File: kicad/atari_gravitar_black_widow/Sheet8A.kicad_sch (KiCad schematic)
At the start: 89 parts, among them Q11 2N3906, Q12 2N3904

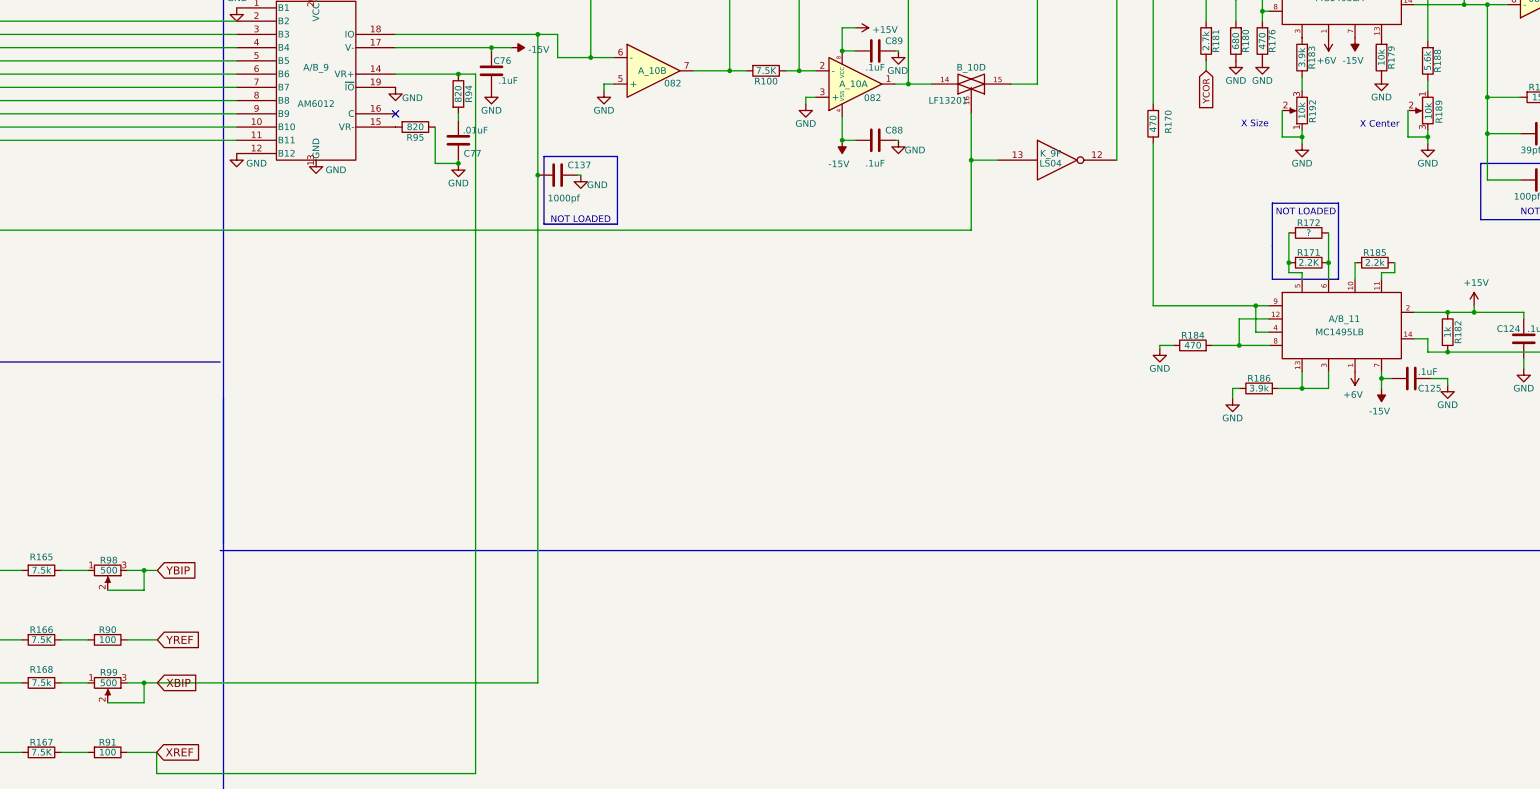
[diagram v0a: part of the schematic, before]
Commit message: Fixed various issues and generated gerber files
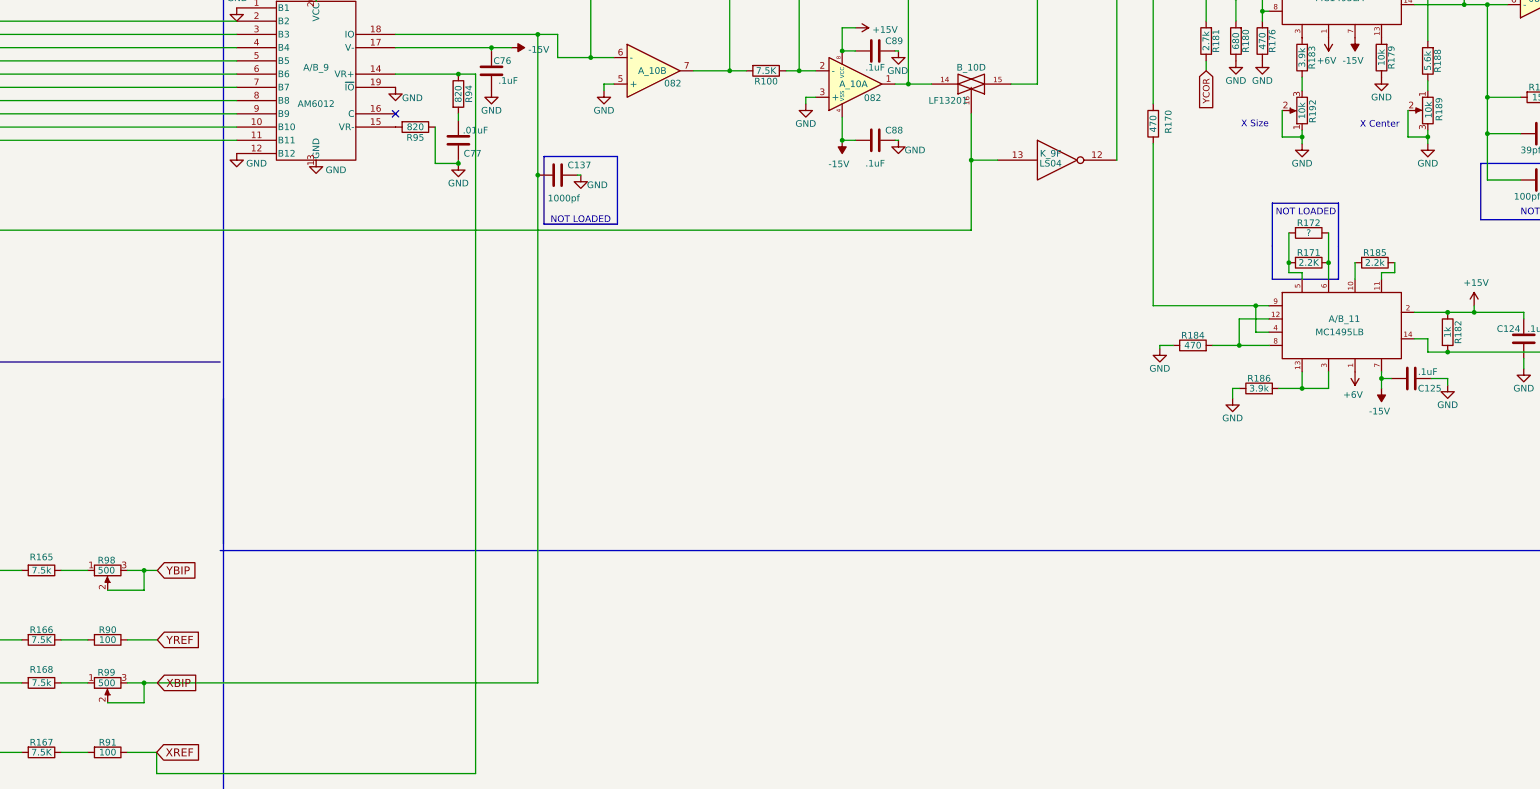
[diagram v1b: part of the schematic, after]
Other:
- moved on the sheet: R189, R98, R99
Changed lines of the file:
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@@
     (pin "1")
   )
-  (symbol (lib_name "POT_4") (lib_id "atari_grav_bw:POT") (at 475.615 104.775 180) (unit 1)
-    (in_bom yes) (on_board yes)
-    (property "Reference" "R189" (id 0) (at 477.7898 107.2797 90)
+  (symbol (lib_id "atari_grav_bw:POT") (at 475.615 104.775 0) (mirror y) (unit 1)
+    (in_bom yes) (on_board yes)
+    (property "Reference" "R189" (id 0) (at 477.7898 102.2703 90)
       (effects (font (size 1.27 1.27)) (justify right))
     )
-    (property "Value" "10k" (id 1) (at 475.7739 106.5044 90)
+    (property "Value" "10k" (id 1) (at 475.7739 103.0456 90)
       (effects (font (size 1.27 1.27)) (justify right))
     )
@@
     (pin "1")
   )
-  (symbol (lib_name "POT_2") (lib_id "atari_grav_bw:POT") (at 222.25 193.04 270) (unit 1)
-    (in_bom yes) (on_board yes)
-    (property "Reference" "R98" (id 0) (at 224.1744 191.109 90)
+  (symbol (lib_id "atari_grav_bw:POT") (at 222.25 193.04 90) (mirror x) (unit 1)
+    (in_bom yes) (on_board yes)
+    (property "Reference" "R98" (id 0) (at 220.3256 191.109 90)
       (effects (font (size 1.27 1.27)) (justify right))
     )
-    (property "Value" "500" (id 1) (at 224.1549 193.0403 90)
+    (property "Value" "500" (id 1) (at 220.3451 193.0403 90)
       (effects (font (size 1.27 1.27)) (justify right))
     )
@@
     (pin "1")
   )
-  (symbol (lib_name "POT_1") (lib_id "atari_grav_bw:POT") (at 222.25 214.63 270) (unit 1)
-    (in_bom yes) (on_board yes)
-    (property "Reference" "R99" (id 0) (at 224.1951 212.6373 90)
+  (symbol (lib_id "atari_grav_bw:POT") (at 222.25 214.63 90) (mirror x) (unit 1)
+    (in_bom yes) (on_board yes)
+    (property "Reference" "R99" (id 0) (at 220.3049 212.6373 90)
       (effects (font (size 1.27 1.27)) (justify right))
     )
-    (property "Value" "500" (id 1) (at 224.0942 214.6542 90)
+    (property "Value" "500" (id 1) (at 220.4058 214.6542 90)
       (effects (font (size 1.27 1.27)) (justify right))
     )
@@
     (pin "2")
   )
-  (symbol (lib_name "POT_3") (lib_id "atari_grav_bw:POT") (at 451.485 104.775 180) (unit 1)
+  (symbol (lib_id "atari_grav_bw:POT") (at 451.485 104.775 180) (unit 1)
     (in_bom yes) (on_board yes)
     (property "Reference" "R192" (id 0) (at 453.517 107.188 90)
